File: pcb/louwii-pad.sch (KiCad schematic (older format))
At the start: 50 parts, among them J1 USB_B_Mini, J2 ICSP, J3 IIC, K1 KEYSW, K2 KEYSW, K3 KEYSW, K4 KEYSW, K5 KEYSW, K6 KEYSW, K7 KEYSW, K8 KEYSW, SW1 SW_Push, U1 ATmega32U4-atmel, X1 16Mhz

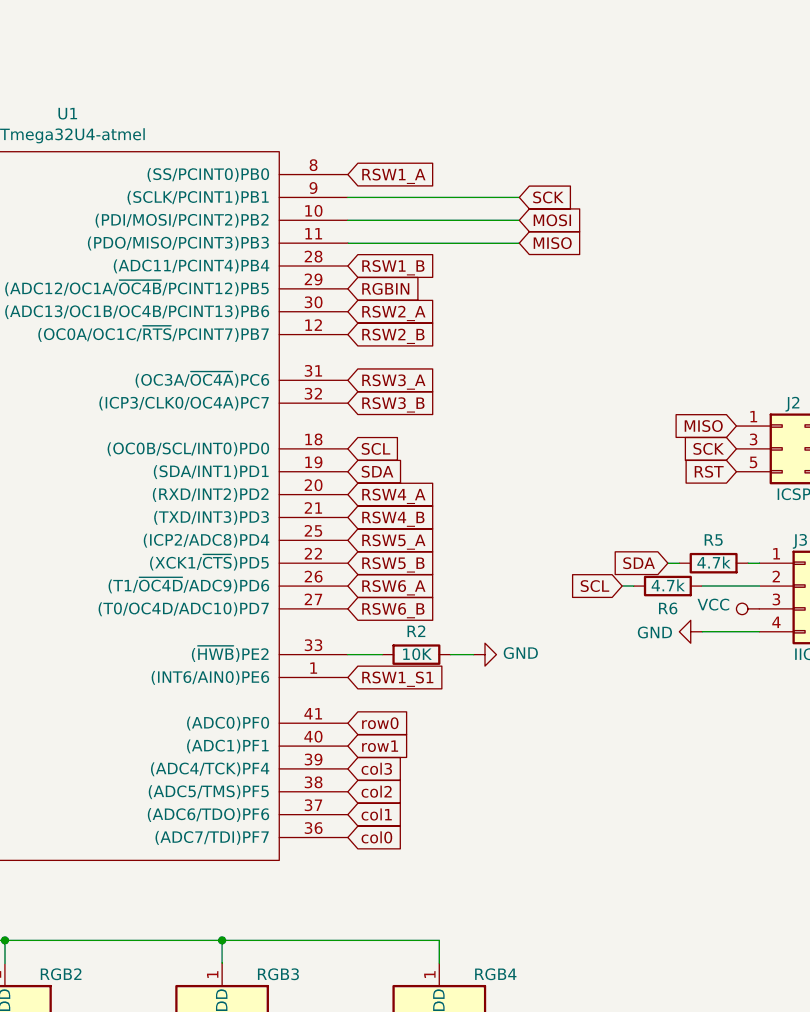
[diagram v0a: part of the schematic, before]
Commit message: add more 3d models, finish up PCB tracing
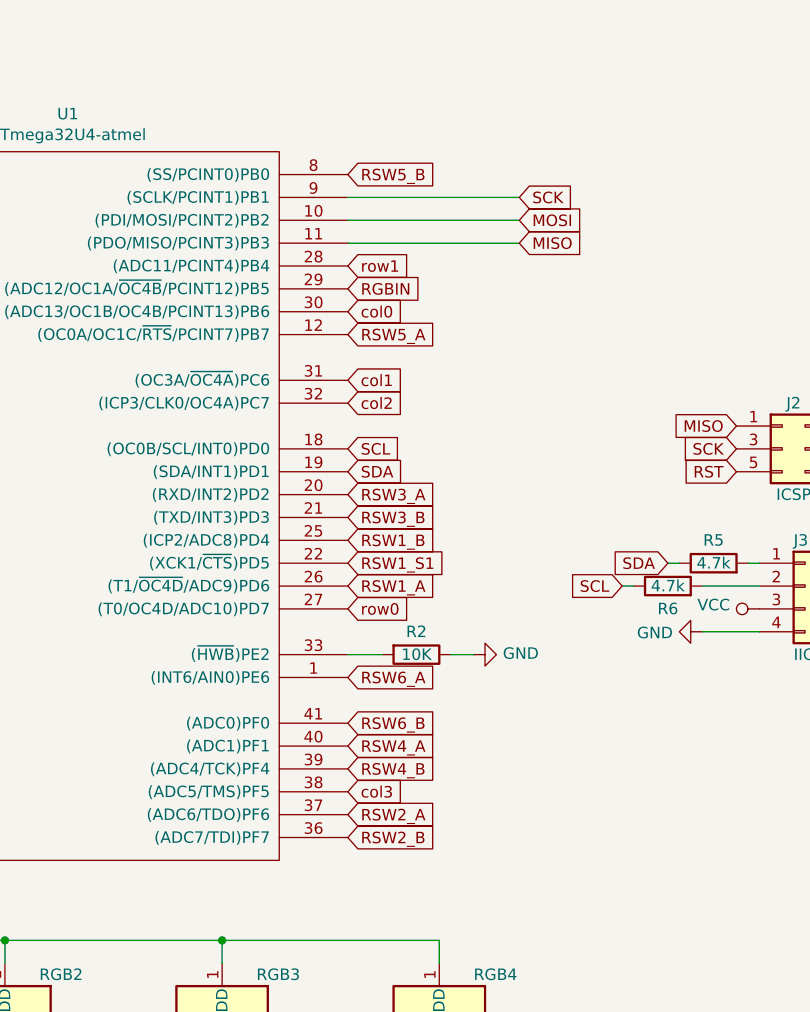
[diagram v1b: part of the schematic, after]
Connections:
- net RSW1_A: now also U1.26 ((T1/~OC4D~/ADC9)PD6); no longer U1.8 ((SS/PCINT0)PB0)
- net RSW1_B: now also U1.25 ((ICP2/ADC8)PD4); no longer U1.28 ((ADC11/PCINT4)PB4)
- net RSW1_S1: now also U1.22 ((XCK1/~CTS~)PD5); no longer U1.1 ((INT6/AIN0)PE6)
- net RSW2_A: now also U1.37 ((ADC6/TDO)PF6); no longer U1.30 ((ADC13/OC1B/OC4B/PCINT13)PB6)
- net RSW2_B: now also U1.36 ((ADC7/TDI)PF7); no longer U1.12 ((OC0A/OC1C/~RTS~/PCINT7)PB7)
- net RSW3_A: now also U1.20 ((RXD/INT2)PD2); no longer U1.31 ((OC3A/~OC4A~)PC6)
- net RSW3_B: now also U1.21 ((TXD/INT3)PD3); no longer U1.32 ((ICP3/CLK0/OC4A)PC7)
- net RSW4_A: now also U1.40 ((ADC1)PF1); no longer U1.20 ((RXD/INT2)PD2)
- net RSW4_B: now also U1.39 ((ADC4/TCK)PF4); no longer U1.21 ((TXD/INT3)PD3)
- net RSW5_A: now also U1.12 ((OC0A/OC1C/~RTS~/PCINT7)PB7); no longer U1.25 ((ICP2/ADC8)PD4)
- net RSW5_B: now also U1.8 ((SS/PCINT0)PB0); no longer U1.22 ((XCK1/~CTS~)PD5)
- net RSW6_A: now also U1.1 ((INT6/AIN0)PE6); no longer U1.26 ((T1/~OC4D~/ADC9)PD6)
- net RSW6_B: now also U1.41 ((ADC0)PF0); no longer U1.27 ((T0/OC4D/ADC10)PD7)
- net col0: now also U1.30 ((ADC13/OC1B/OC4B/PCINT13)PB6); no longer U1.36 ((ADC7/TDI)PF7)
- net col1: now also U1.31 ((OC3A/~OC4A~)PC6); no longer U1.37 ((ADC6/TDO)PF6)
- net col2: now also U1.32 ((ICP3/CLK0/OC4A)PC7); no longer U1.38 ((ADC5/TMS)PF5)
- net col3: now also U1.38 ((ADC5/TMS)PF5); no longer U1.39 ((ADC4/TCK)PF4)
- net row0: now also U1.27 ((T0/OC4D/ADC10)PD7); no longer U1.41 ((ADC0)PF0)
- net row1: now also U1.28 ((ADC11/PCINT4)PB4); no longer U1.40 ((ADC1)PF1)
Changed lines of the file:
@@
 	1    0    0    -1
 $EndComp
-Text GLabel 5050 1500 2    50   Input ~ 0
+Text GLabel 5050 3300 2    50   Input ~ 0
 RSW1_A
-Text GLabel 5050 1900 2    50   Input ~ 0
+Text GLabel 5050 3100 2    50   Input ~ 0
 RSW1_B
 Text GLabel 9750 1850 0    50   Input ~ 0
@@
 Text GLabel 9750 2050 0    50   Input ~ 0
 RSW1_B
-Text GLabel 5050 2100 2    50   Input ~ 0
+Text GLabel 5050 4300 2    50   Input ~ 0
 RSW2_A
-Text GLabel 5050 2200 2    50   Input ~ 0
+Text GLabel 5050 4400 2    50   Input ~ 0
 RSW2_B
-Text GLabel 5050 2400 2    50   Input ~ 0
+Text GLabel 5050 2900 2    50   Input ~ 0
 RSW3_A
-Text GLabel 5050 2500 2    50   Input ~ 0
+Text GLabel 5050 3000 2    50   Input ~ 0
 RSW3_B
-Text GLabel 5050 2900 2    50   Input ~ 0
+Text GLabel 5050 4000 2    50   Input ~ 0
 RSW4_A
-Text GLabel 5050 3000 2    50   Input ~ 0
+Text GLabel 5050 4100 2    50   Input ~ 0
 RSW4_B
 Connection ~ 9250 4050
@@
 Text GLabel 9750 4850 0    50   Input ~ 0
 RSW5_B
-Text GLabel 5050 3100 2    50   Input ~ 0
+Text GLabel 5050 2200 2    50   Input ~ 0
 RSW5_A
-Text GLabel 5050 3200 2    50   Input ~ 0
+Text GLabel 5050 1500 2    50   Input ~ 0
 RSW5_B
 Wire Wire Line
@@
 Text GLabel 9750 5550 0    50   Input ~ 0
 RSW6_B
-Text GLabel 5050 3300 2    50   Input ~ 0
+Text GLabel 5050 3700 2    50   Input ~ 0
 RSW6_A
-Text GLabel 5050 3400 2    50   Input ~ 0
+Text GLabel 5050 3900 2    50   Input ~ 0
 RSW6_B
 $Comp
@@
 	2000 6450 2000 6100
 Connection ~ 2000 6450
-Text GLabel 5050 3900 2    50   Input ~ 0
+Text GLabel 5050 3400 2    50   Input ~ 0
 row0
-Text GLabel 5050 4000 2    50   Input ~ 0
+Text GLabel 5050 1900 2    50   Input ~ 0
 row1
-Text GLabel 5050 4400 2    50   Input ~ 0
+Text GLabel 5050 2100 2    50   Input ~ 0
 col0
+Text GLabel 5050 2500 2    50   Input ~ 0
+col2
+Text GLabel 5050 2400 2    50   Input ~ 0
+col1
 Text GLabel 5050 4200 2    50   Input ~ 0
-col2
-Text GLabel 5050 4300 2    50   Input ~ 0
-col1
-Text GLabel 5050 4100 2    50   Input ~ 0
 col3
 Text GLabel 5050 2700 2    50   Input ~ 0
@@
 Wire Wire Line
 	10600 2050 10350 2050
-Text GLabel 5050 3700 2    50   Input ~ 0
+Text GLabel 5050 3200 2    50   Input ~ 0
 RSW1_S1
 $Comp
